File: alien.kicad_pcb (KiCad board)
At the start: 2 copper layers, 49 parts, among them Q1 2N3904, Q2 2N3904, Q3 2N5457, U1 LM324, X1 JD_CONN_01X01, X10 JD_CONN_01X01, X11 JD_CONN_01X01, X12 JD_CONN_01X02, X13 JD_CONN_01X02, X2 JD_CONN_01X01, X3 JD_CONN_01X01, X4 JD_CONN_01X01, X5 JD_CONN_01X01, X6 JD_CONN_01X01, X7 JD_CONN_01X01, X8 JD_CONN_01X01, X9 JD_CONN_01X01

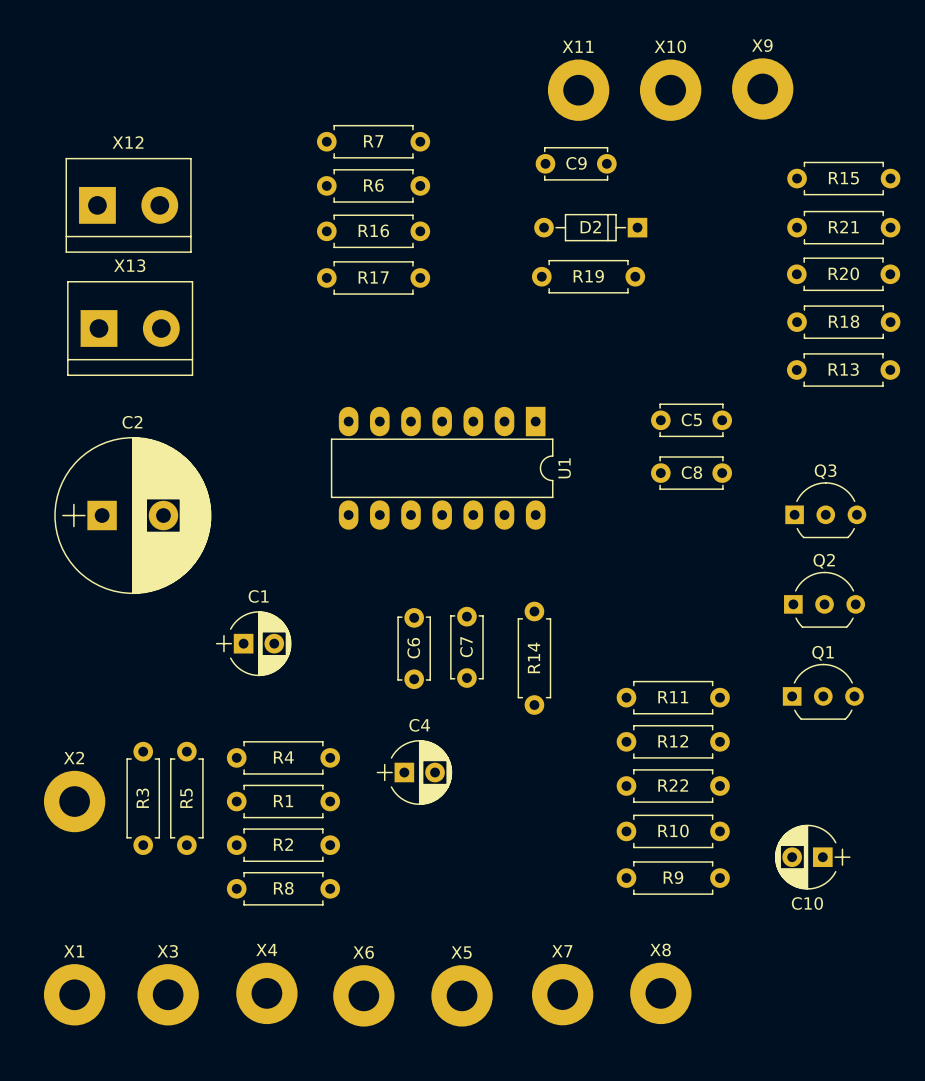
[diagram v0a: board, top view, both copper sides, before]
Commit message: empezamos a enrutar
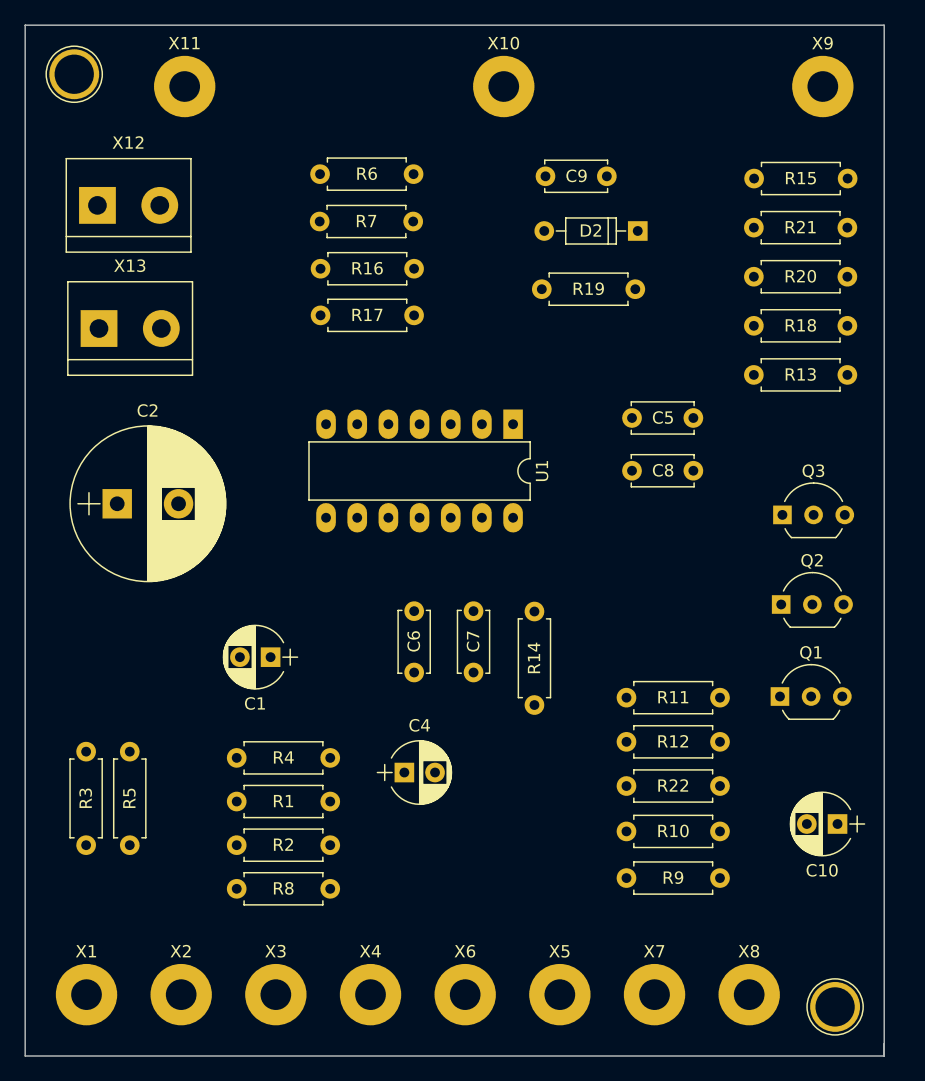
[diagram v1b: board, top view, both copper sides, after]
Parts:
- added REF**: 1pin, Connectors:1pin, F.Cu at (138.0, 144.0)
- added REF**: 1pin, Connectors:1pin, F.Cu at (76.0, 68.0)
- moved X11 32.1 mm to (85.0, 69.0)
- moved X2 18.0 mm to (84.7, 143.0)
- moved X10 13.6 mm to (111.0, 69.0)
- moved R7 10.5 mm to (96.0, 80.0), turned to 0 degrees
- moved X3 8.78 mm to (92.4, 143.0)
- moved X4 8.44 mm to (100.1, 143.0)
- moved X6 8.26 mm to (107.9, 143.0)
- moved X5 7.97 mm to (115.6, 143.0)
- moved X7 7.49 mm to (123.3, 143.0)
- moved X8 7.20 mm to (131.0, 143.0)
- moved X9 4.90 mm to (137.0, 69.0)
- moved R3 4.65 mm to (77.0, 130.8)
- moved R5 4.65 mm to (80.5, 130.8)
- moved R18 4.11 mm to (139.0, 88.5), turned to 180 degrees
- moved R21 4.10 mm to (139.0, 80.5), turned to 180 degrees
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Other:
- board outline added: 70 x 84 mm
- net class sinte added: clearance 0.5, trace_width 0.8, via_dia 0.6, via_drill 0.4
